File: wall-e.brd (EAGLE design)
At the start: 62.3 x 52.7 mm, 71 parts, among them IC1 VREG-TS1117CW-3V3, T1 BC847, U1 TSM2306CX, U2 TSM2306CX, U3 TSM2306CX, U4 TSM2306CX, U5 TSM2306CX, U6 TSM2306CX, U7 TSM2306CX, U8 LM293AD, U9 TSM2306CX

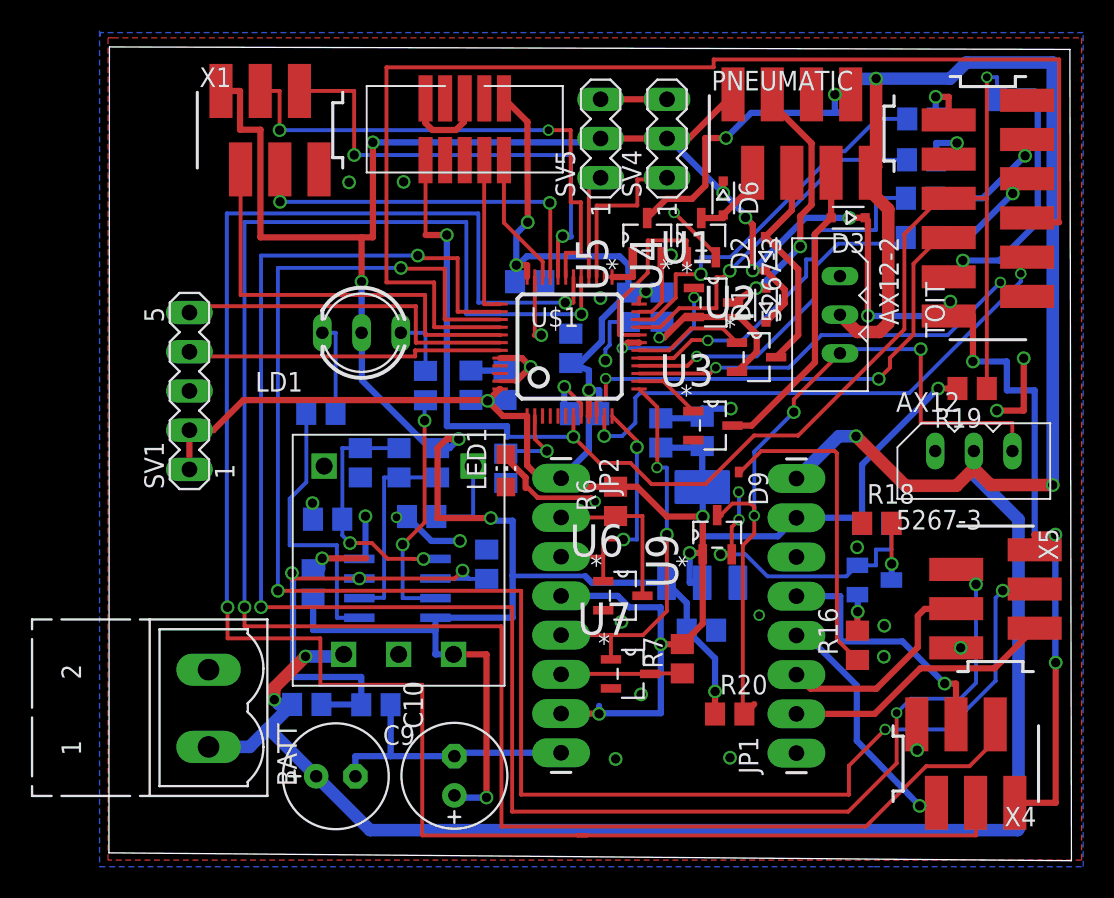
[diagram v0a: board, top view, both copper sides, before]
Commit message: Some corrections
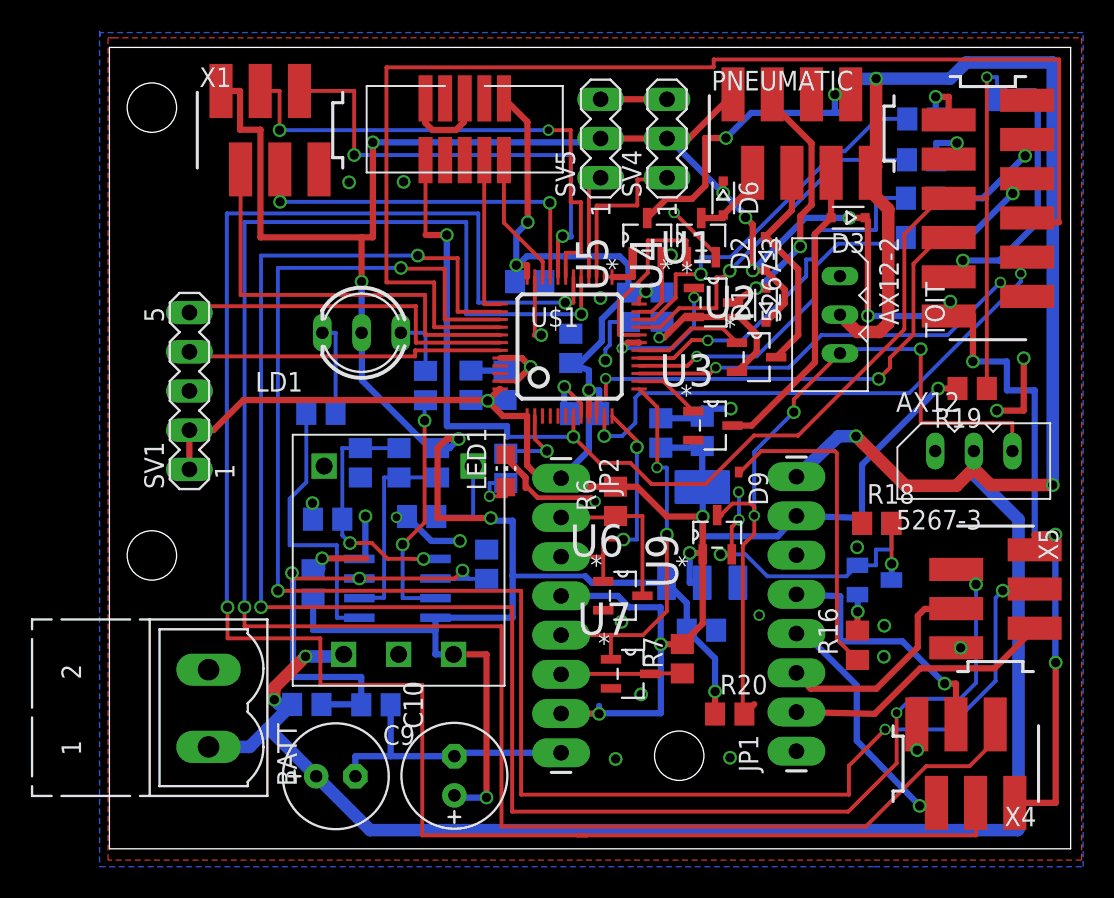
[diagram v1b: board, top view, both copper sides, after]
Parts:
- moved JP1 0.12 mm to (97.2, 23.3)
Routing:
- net N$18: track 0.00 -> 3.57 mm, vias 0 -> 1
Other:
- board size 62.3 x 52.7 mm -> 62.2 x 51.9 mm
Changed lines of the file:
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@@
 <layer number="43" name="vRestrict" color="2" fill="10" visible="yes" active="yes"/>
 <layer number="44" name="Drills" color="7" fill="1" visible="no" active="yes"/>
-<layer number="45" name="Holes" color="7" fill="1" visible="no" active="yes"/>
+<layer number="45" name="Holes" color="7" fill="1" visible="yes" active="yes"/>
 <layer number="46" name="Milling" color="3" fill="1" visible="no" active="yes"/>
 <layer number="47" name="Measures" color="7" fill="1" visible="no" active="yes"/>
@@
 <board>
 <plain>
-<wire x1="52.72" y1="16.74" x2="115.05" y2="16.23" width="0" layer="20"/>
-<wire x1="115.05" y1="16.23" x2="114.95" y2="68.77" width="0" layer="20"/>
-<wire x1="114.95" y1="68.77" x2="52.75" y2="68.93" width="0" layer="20"/>
-<wire x1="52.75" y1="68.93" x2="52.72" y2="16.74" width="0" layer="20"/>
+<wire x1="52.75" y1="17" x2="115" y2="17" width="0" layer="20"/>
+<wire x1="115" y1="17" x2="115" y2="68.9" width="0" layer="20"/>
+<wire x1="115" y1="68.9" x2="52.75" y2="68.9" width="0" layer="20"/>
+<wire x1="52.75" y1="68.9" x2="52.75" y2="17" width="0" layer="20"/>
+<hole x="55.5" y="65" drill="3.2"/>
+<hole x="55.5" y="36" drill="3.2"/>
+<hole x="89.65" y="23.03" drill="3.2"/>
 </plain>
 <attributes>
@@
 </element>
 <element name="X1" library="con-amp" package="SMDTOP6" value="" x="63.15" y="63.54"/>
-<element name="JP1" library="SparkFun" package="1X08_LONGPADS" value="" x="97.24" y="23.2" rot="R90"/>
+<element name="JP1" library="SparkFun" package="1X08_LONGPADS" value="" x="97.24" y="23.32" rot="R90"/>
 <element name="JP2" library="SparkFun" package="1X08_LONGPADS" value="" x="82" y="41" rot="R270"/>
 <element name="X4" library="con-amp" package="SMDTOP6" value="" x="108.21" y="22.52" rot="R180"/>
@@
 <wire x1="83.8" y1="47.99" x2="82.63" y2="48.46" width="0.4064" layer="16"/>
 <wire x1="83.8" y1="47.99" x2="83.8" y2="46.7" width="0.4064" layer="16"/>
-<wire x1="101.12" y1="38.44" x2="97.24" y2="38.44" width="0.4064" layer="16"/>
+<wire x1="101.12" y1="38.44" x2="97.24" y2="38.56" width="0.4064" layer="16"/>
 <wire x1="101.12" y1="38.44" x2="101.49" y2="38.07" width="0.4064" layer="16"/>
 <wire x1="101.49" y1="38.07" x2="101.49" y2="41.88" width="0.4064" layer="16"/>
@@
 <wire x1="91.14" y1="40.429" x2="91.1702" y2="40.429" width="0.4064" layer="16"/>
 <wire x1="91.1702" y1="38.52" x2="91.1702" y2="40.429" width="0.4064" layer="16"/>
-<wire x1="97.24" y1="38.44" x2="96.04" y2="37.24" width="0.4064" layer="16"/>
+<wire x1="97.24" y1="38.56" x2="96.04" y2="37.24" width="0.4064" layer="16"/>
 <wire x1="96.04" y1="37.24" x2="91.1702" y2="37.24" width="0.4064" layer="16"/>
 <wire x1="91.1702" y1="37.24" x2="91.1702" y2="38.52" width="0.4064" layer="16"/>
@@
 <wire x1="111.62" y1="38.34" x2="108.73" y2="41.23" width="0.8128" layer="16"/>
 <wire x1="108.73" y1="41.23" x2="108.73" y2="42.76" width="0.8128" layer="16"/>
-<wire x1="97.24" y1="40.98" x2="99.98" y2="43.72" width="0.8128" layer="16"/>
+<wire x1="97.24" y1="41.1" x2="99.98" y2="43.72" width="0.8128" layer="16"/>
 <wire x1="99.98" y1="43.72" x2="101.1" y2="43.72" width="0.8128" layer="16"/>
 <via x="101.1" y="43.72" extent="1-16" drill="0.6" shape="square"/>
@@
 <wire x1="106.84" y1="27.7" x2="104.11" y2="30.43" width="0.4064" layer="16"/>
 <wire x1="100.08" y1="30.43" x2="104.11" y2="30.43" width="0.4064" layer="16"/>
-<wire x1="97.24" y1="33.27" x2="97.24" y2="33.36" width="0.4064" layer="16"/>
-<wire x1="97.24" y1="33.36" x2="100.08" y2="33.36" width="0.4064" layer="16"/>
+<wire x1="97.24" y1="33.27" x2="97.24" y2="33.48" width="0.4064" layer="16"/>
+<wire x1="97.24" y1="33.48" x2="100.08" y2="33.36" width="0.4064" layer="16"/>
 <wire x1="100.08" y1="33.36" x2="100.08" y2="30.43" width="0.4064" layer="16"/>
 </signal>
@@
 <wire x1="101.15" y1="24" x2="101.15" y2="27.58" width="0.4064" layer="16"/>
 <wire x1="101.15" y1="27.58" x2="97.91" y2="30.82" width="0.4064" layer="16"/>
-<wire x1="97.91" y1="30.82" x2="97.24" y2="30.82" width="0.4064" layer="16"/>
+<wire x1="97.91" y1="30.82" x2="97.24" y2="30.94" width="0.4064" layer="16"/>
 <wire x1="106.305" y1="19.98" x2="106.305" y2="19.78" width="0.4064" layer="1"/>
 <wire x1="106.305" y1="19.78" x2="105.22" y2="19.78" width="0.4064" layer="1"/>
@@
 <wire x1="105.55" y1="32.54" x2="107.575" y2="32.54" width="0.4064" layer="1"/>
 <wire x1="107.575" y1="32.54" x2="107.59" y2="32.555" width="0.4064" layer="1"/>
-<wire x1="97.24" y1="28.28" x2="98.15" y2="27.37" width="0.4064" layer="1"/>
+<wire x1="97.24" y1="28.4" x2="98.15" y2="27.37" width="0.4064" layer="1"/>
 <wire x1="98.15" y1="27.37" x2="102.42" y2="27.37" width="0.4064" layer="1"/>
 <wire x1="102.42" y1="27.37" x2="105.1" y2="30.05" width="0.4064" layer="1"/>
@@
 <contactref element="JP1" pad="2"/>
 <contactref element="X5" pad="5"/>
-<wire x1="97.24" y1="25.74" x2="102.31" y2="25.74" width="0.4064" layer="1"/>
+<wire x1="97.24" y1="25.86" x2="102.31" y2="25.74" width="0.4064" layer="1"/>
 <wire x1="102.31" y1="25.74" x2="105.26" y2="28.69" width="0.4064" layer="1"/>
 <wire x1="105.26" y1="28.69" x2="110.075" y2="28.69" width="0.4064" layer="1"/>
@@
 <contactref element="R1" pad="2"/>
 <contactref element="LED1" pad="A"/>
-<wire x1="78.43" y1="40.43" x2="78.42" y2="40.69" width="0" layer="19" extent="1-16"/>
+<wire x1="78.42" y1="40.69" x2="77.37" y2="40.69" width="0.254" layer="16"/>
+<wire x1="77.37" y1="40.69" x2="77.37" y2="39.83" width="0.254" layer="16"/>
+<via x="77.37" y="39.83" extent="1-16" drill="0.5" shape="square"/>
+<wire x1="77.37" y1="39.83" x2="78.43" y2="39.83" width="0.254" layer="1"/>
+<wire x1="78.43" y1="39.83" x2="78.43" y2="40.43" width="0.254" layer="1"/>
 </signal>
 <signal name="N$22">
